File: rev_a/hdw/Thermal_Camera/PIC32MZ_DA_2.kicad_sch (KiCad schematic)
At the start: 1 part

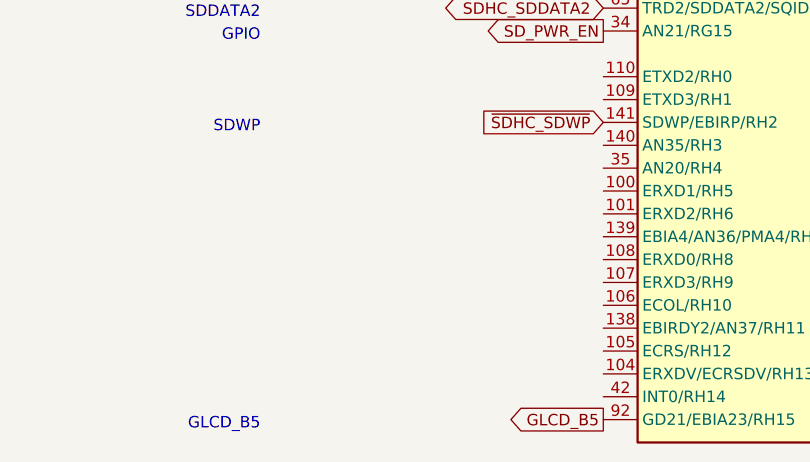
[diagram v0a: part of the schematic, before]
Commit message: blah blah
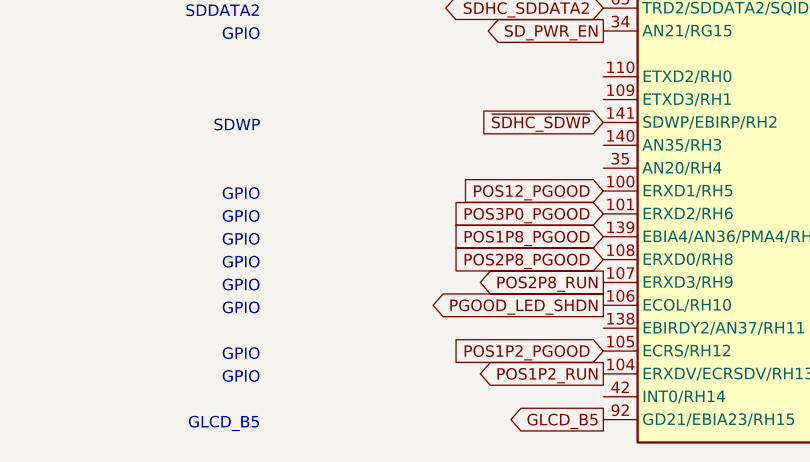
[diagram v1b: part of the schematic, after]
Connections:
- net POS12_PGOOD: now reaches U?.100 (ERXD1/RH5)
- net POS3P0_PGOOD: now reaches U?.101 (ERXD2/RH6)
- net POS1P2_RUN: now reaches U?.104 (ERXDV/ECRSDV/RH13)
- net POS1P2_PGOOD: now reaches U?.105 (ECRS/RH12)
- net PGOOD_LED_SHDN: now reaches U?.106 (ECOL/RH10)
- net POS2P8_RUN: now reaches U?.107 (ERXD3/RH9)
- net POS2P8_PGOOD: now reaches U?.108 (ERXD0/RH8)
- net POS1P8_PGOOD: now reaches U?.139 (EBIA4/AN36/PMA4/RH7)
